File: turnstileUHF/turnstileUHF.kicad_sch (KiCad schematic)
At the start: 54 parts, among them J5 RFPC-SMA28-F, Q1 2N7002, Q2 2N7002, Q3 2N7002, Q4 2N7002, Q5 AO3401A, Q6 AO3401A, Q7 AO3401A, Q8 2N7002, U1 74HCT238D

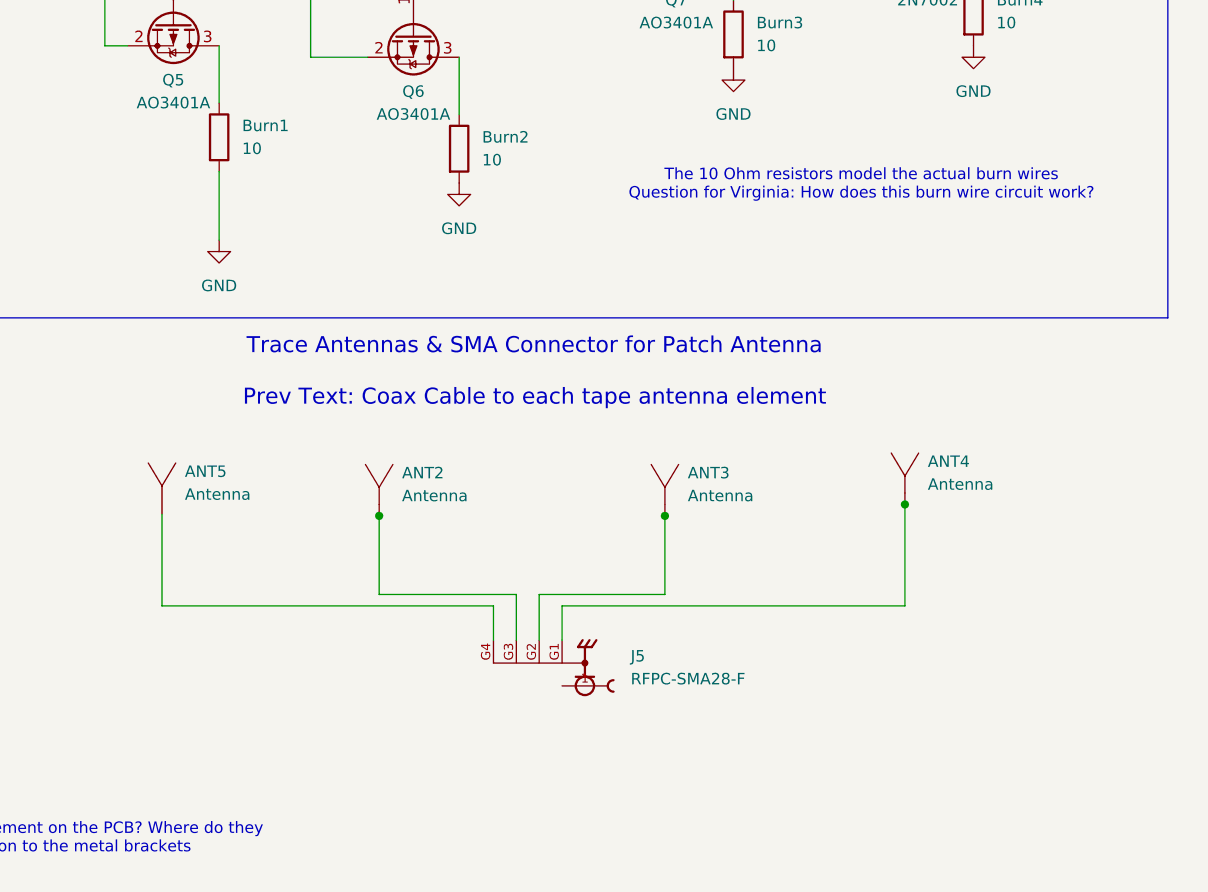
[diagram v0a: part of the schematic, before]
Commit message: Meeting changes 09-25-2026
Changes made to the schematic, ready to be routed
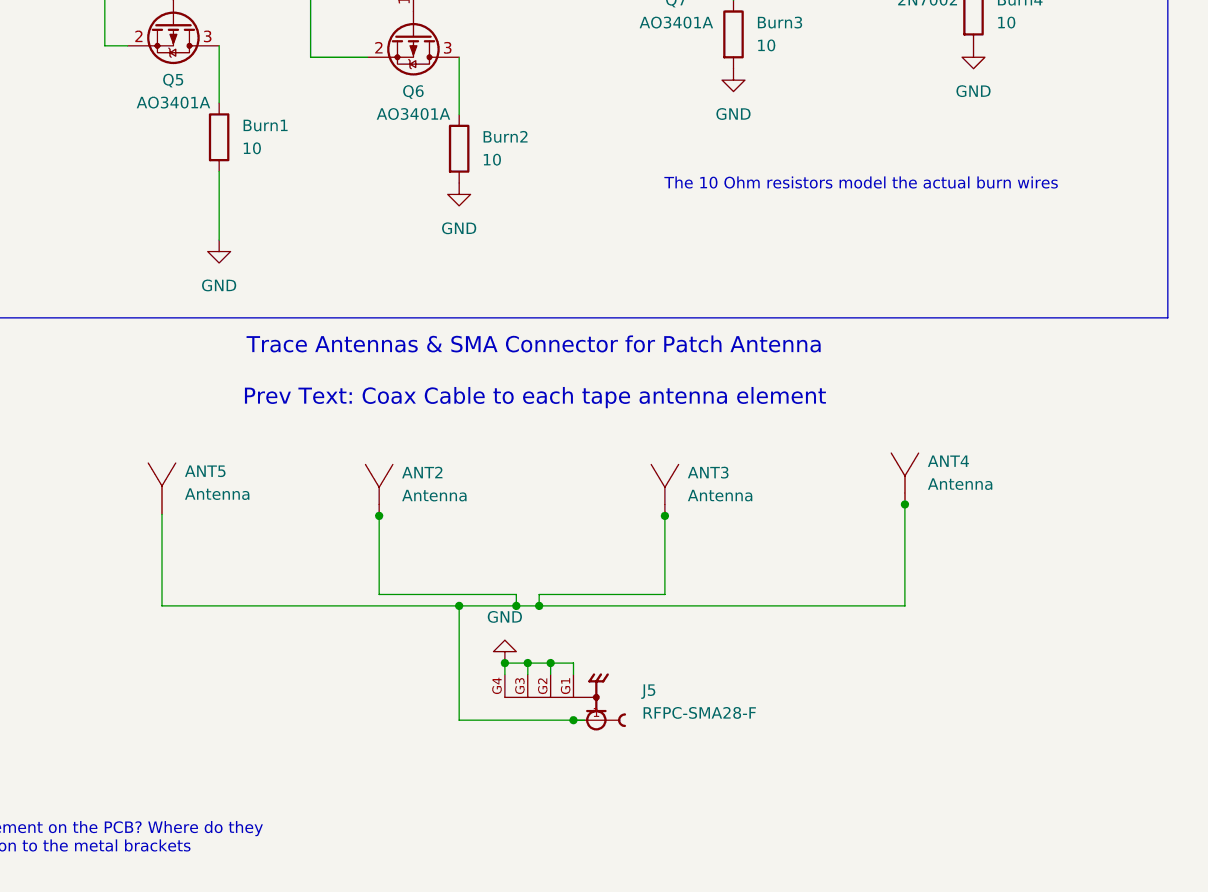
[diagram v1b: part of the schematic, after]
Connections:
- net GND: now also J5.G1, J5.G2, J5.G3, J5.G4
- net at J5.1: now also ANT2.1, ANT3.1, ANT4.1, ANT5.1
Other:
- note added: "The 10 Ohm resistors model the actual burn wires"
- note removed: "The 10 Ohm resistors model the actual burn wires Question for Virginia: How does this burn wire circuit work?"
- moved on the sheet: J5
